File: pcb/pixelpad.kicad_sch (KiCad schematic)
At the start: 16 parts, among them SW1 SW_Push_45deg, SW2 SW_Push_45deg, SW3 SW_Push_45deg, SW4 SW_Push_45deg, SW5 SW_Push_45deg, SW6 RotaryEncoder_Switch, U1 MOUDLE-SEEEDUINO-XIAO, U2 ER_OLEDM0.91_1x-I2C

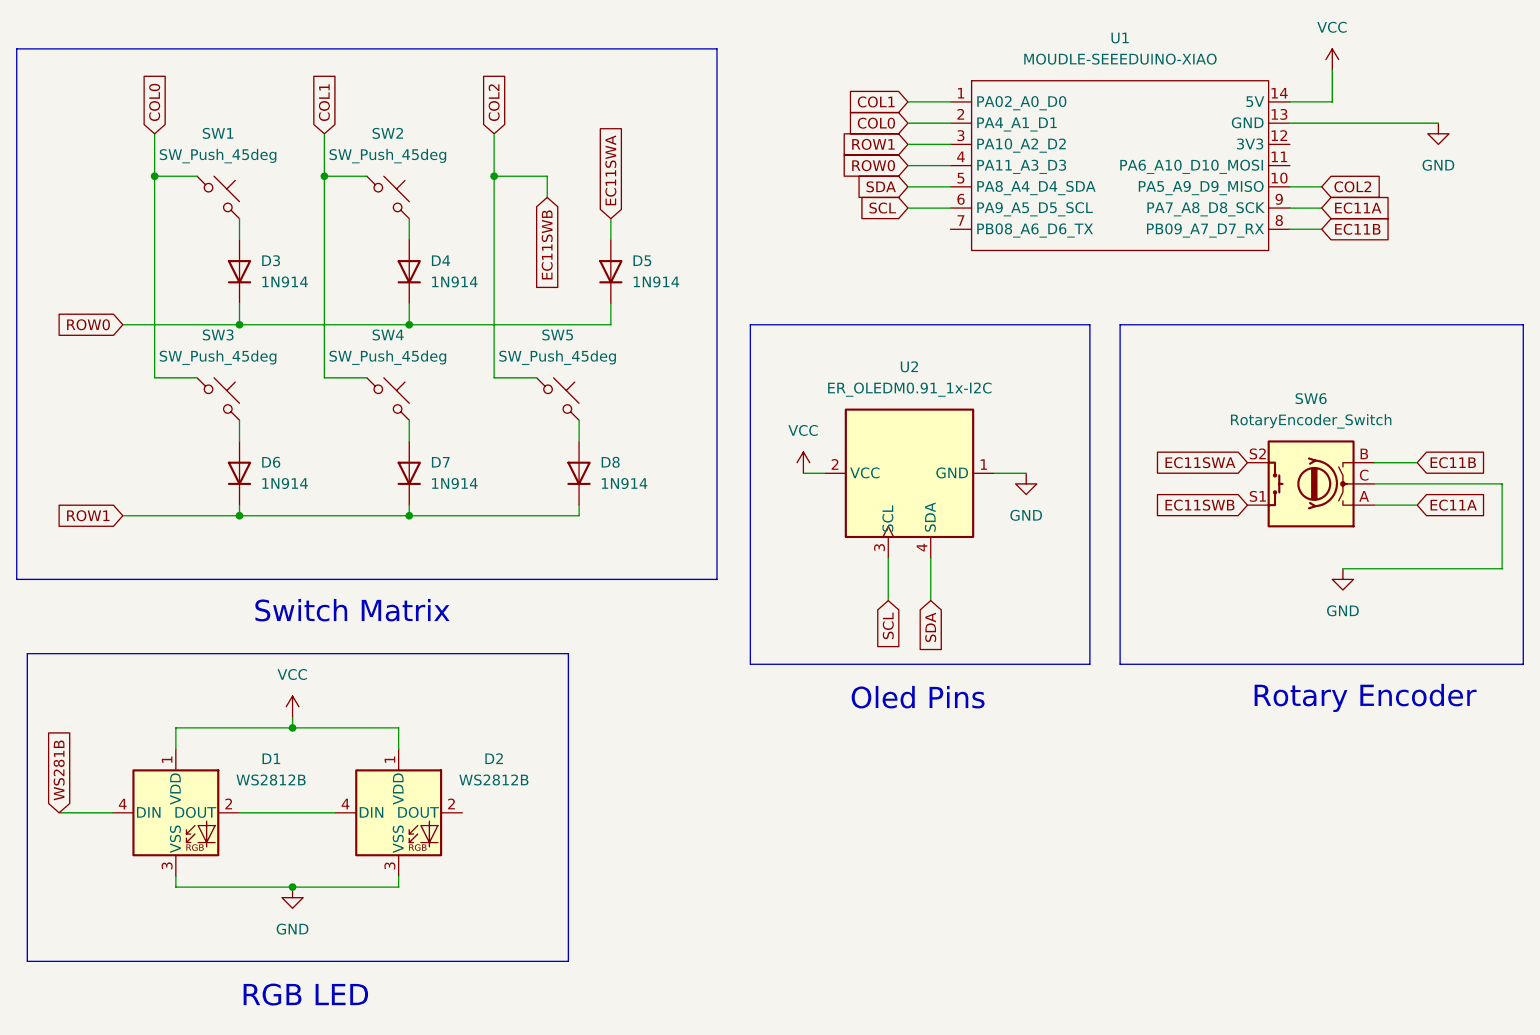
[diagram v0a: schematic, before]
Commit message: Reordered
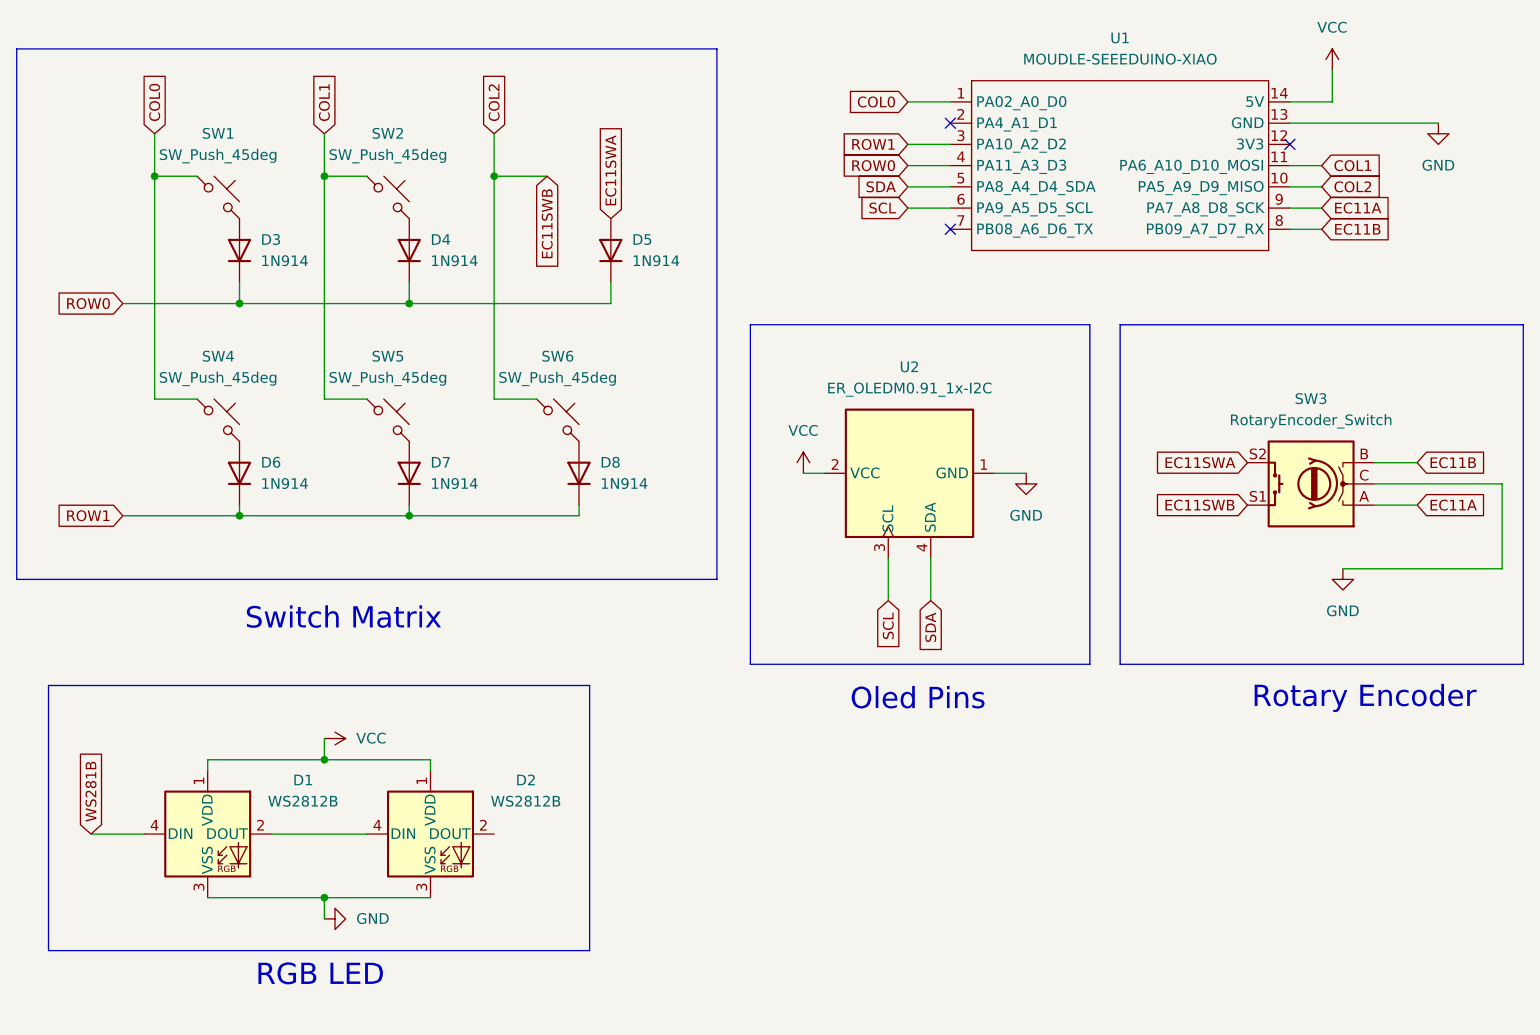
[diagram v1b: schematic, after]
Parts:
- removed SW3: SW_Push_45deg, Button_Switch_Keyboard:SW_Cherry_MX_1.00u_PCB, symbol KiCad-User:SW_Push_45deg
- added SW6: SW_Push_45deg, Button_Switch_Keyboard:SW_Cherry_MX_1.00u_PCB, symbol KiCad-User:SW_Push_45deg
- renumbered SW6 to SW3
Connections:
- net COL0: now also SW4.1, U1.1 (PA02_A0_D0); no longer U1.2 (PA4_A1_D1)
- net COL1: now also SW5.1, U1.11 (PA6_A10_D10_MOSI); no longer SW4.1, U1.1 (PA02_A0_D0)
- net COL2: now also SW6.1; no longer SW5.1
- net at D6.2 (A): now also SW4.2
- net at D7.2 (A): now also SW5.2; no longer SW4.2
- net at D8.2 (A): now also SW6.2; no longer SW5.2
- no-connect marks 0 -> 3
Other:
- moved on the sheet: D1, D2
